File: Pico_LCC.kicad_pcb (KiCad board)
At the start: 2 copper layers, 85 x 100 mm, 77 parts, among them J1 Screw_Terminal_01x12, J2 RJHSE508002, J3 SM04B-SRSS-TB, J4 SM04B-SRSS-TB, U1 SN3257QPWRQ1, U10 SN74HC253DR, U11 DRV8874PWPR, U12 6N137, U13 6N137, U2 MCP2562-E-SN, U4 SN74HC253DR, U5 DRV8874PWPR, U6 SN74HC253DR, U7 DRV8874PWPR, U8 SN74HC253DR, U9 DRV8874PWPR

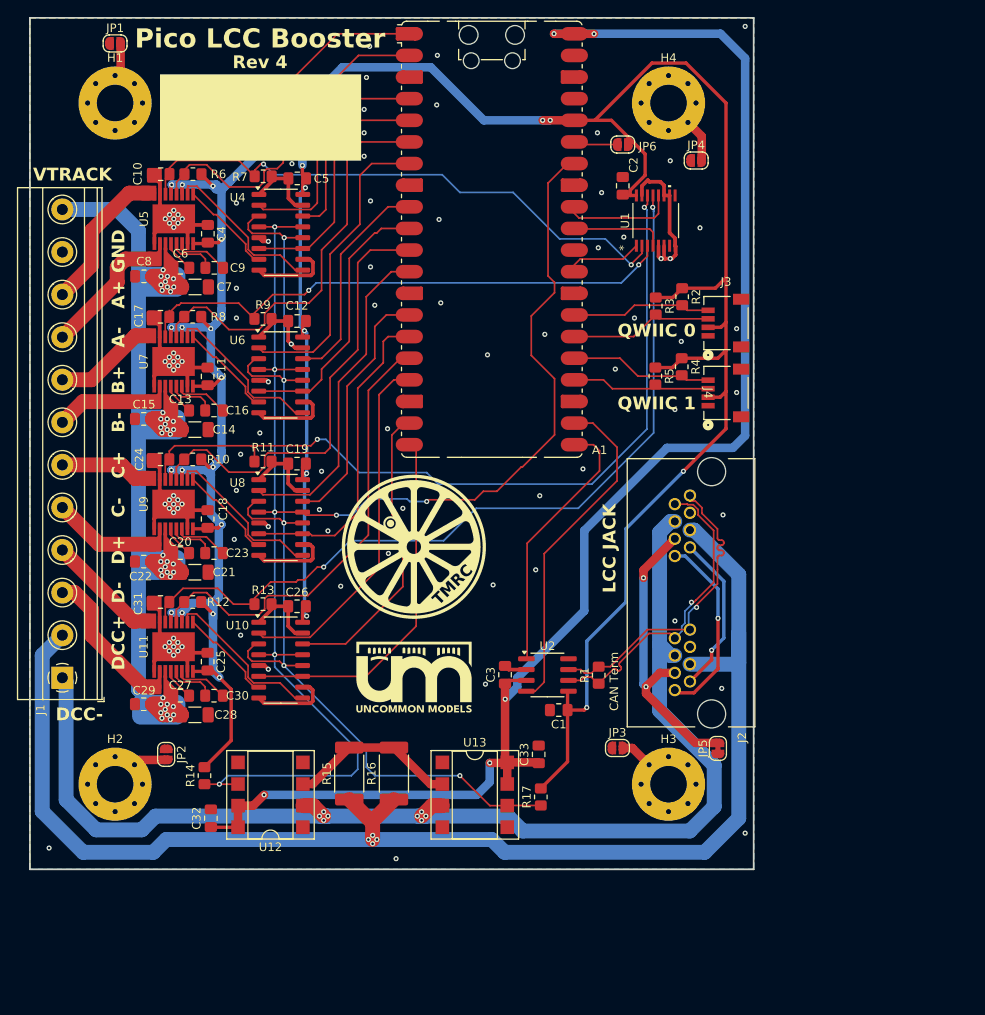
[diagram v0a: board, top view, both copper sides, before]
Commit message: v4 with Stencil and Frame
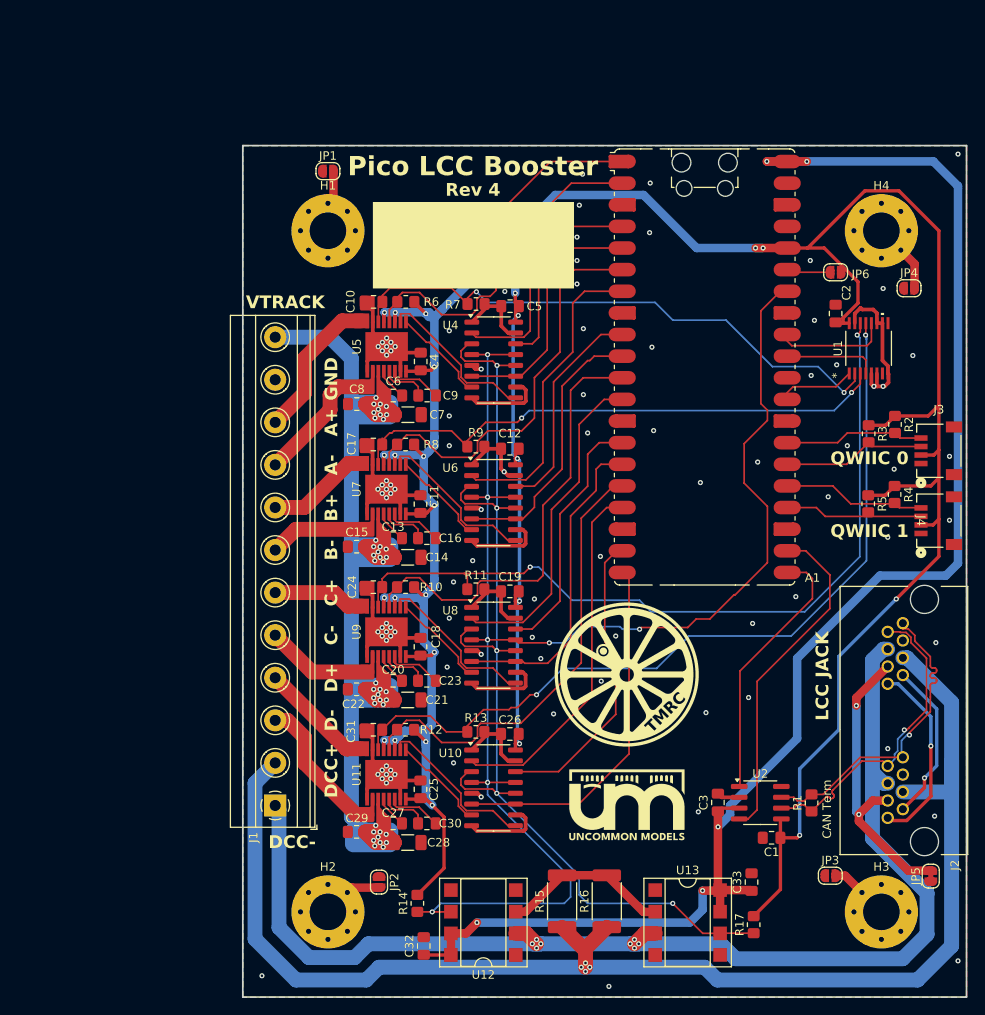
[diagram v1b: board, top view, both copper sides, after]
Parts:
- moved JP5 29.2 mm to (130.8, 125.8)
- moved C17 29.2 mm to (65.3, 75.1)
- moved C24 29.2 mm to (65.3, 91.9)
- moved C31 29.2 mm to (65.3, 108.6)
- moved C6 29.2 mm to (67.7, 69.4)
- moved A1 29.2 mm to (104.2, 66.0)
- moved C1 29.2 mm to (112.1, 121.3)
- moved C10 29.2 mm to (65.4, 58.4)
- moved C11 29.2 mm to (70.9, 82.1)
- moved C12 29.2 mm to (81.4, 75.6)
- moved C14 29.2 mm to (69.4, 88.4)
- moved C15 29.2 mm to (63.4, 87.1)
- moved C16 29.2 mm to (71.6, 86.1)
- moved C18 29.2 mm to (70.9, 98.9)
- moved C19 29.2 mm to (81.4, 92.4)
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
